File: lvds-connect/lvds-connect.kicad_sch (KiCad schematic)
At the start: 2 parts, among them J1 Conn_02x15_Odd_Even, J2 Conn_01x22

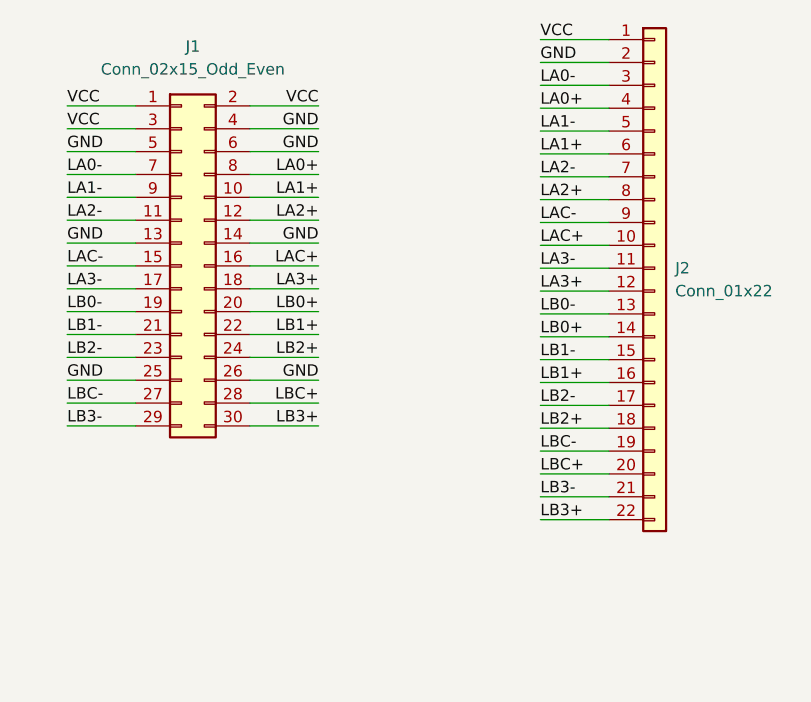
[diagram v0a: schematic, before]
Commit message: 도면 태그 기입
Signed-off-by: Ju, Gyeong-min <jcmh74@gmail.com>
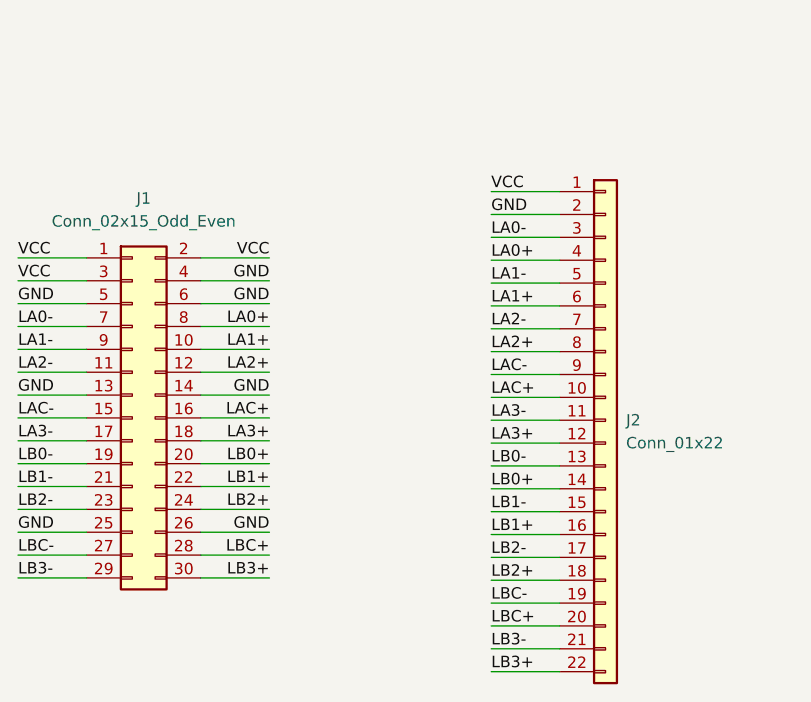
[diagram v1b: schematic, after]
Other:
- company: (none) -> Amos Home
- title: (none) -> LVDS Connector
- moved on the sheet: J1, J2
